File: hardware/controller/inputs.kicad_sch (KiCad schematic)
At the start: 19 parts, among them SW1 EVP-ASAC1A, SW2 EVP-ASAC1A, SW3 EVP-ASAC1A, SW4 EVP-ASAC1A, SW5 EVP-ASAC1A, SW6 CL-SB-13A-02T

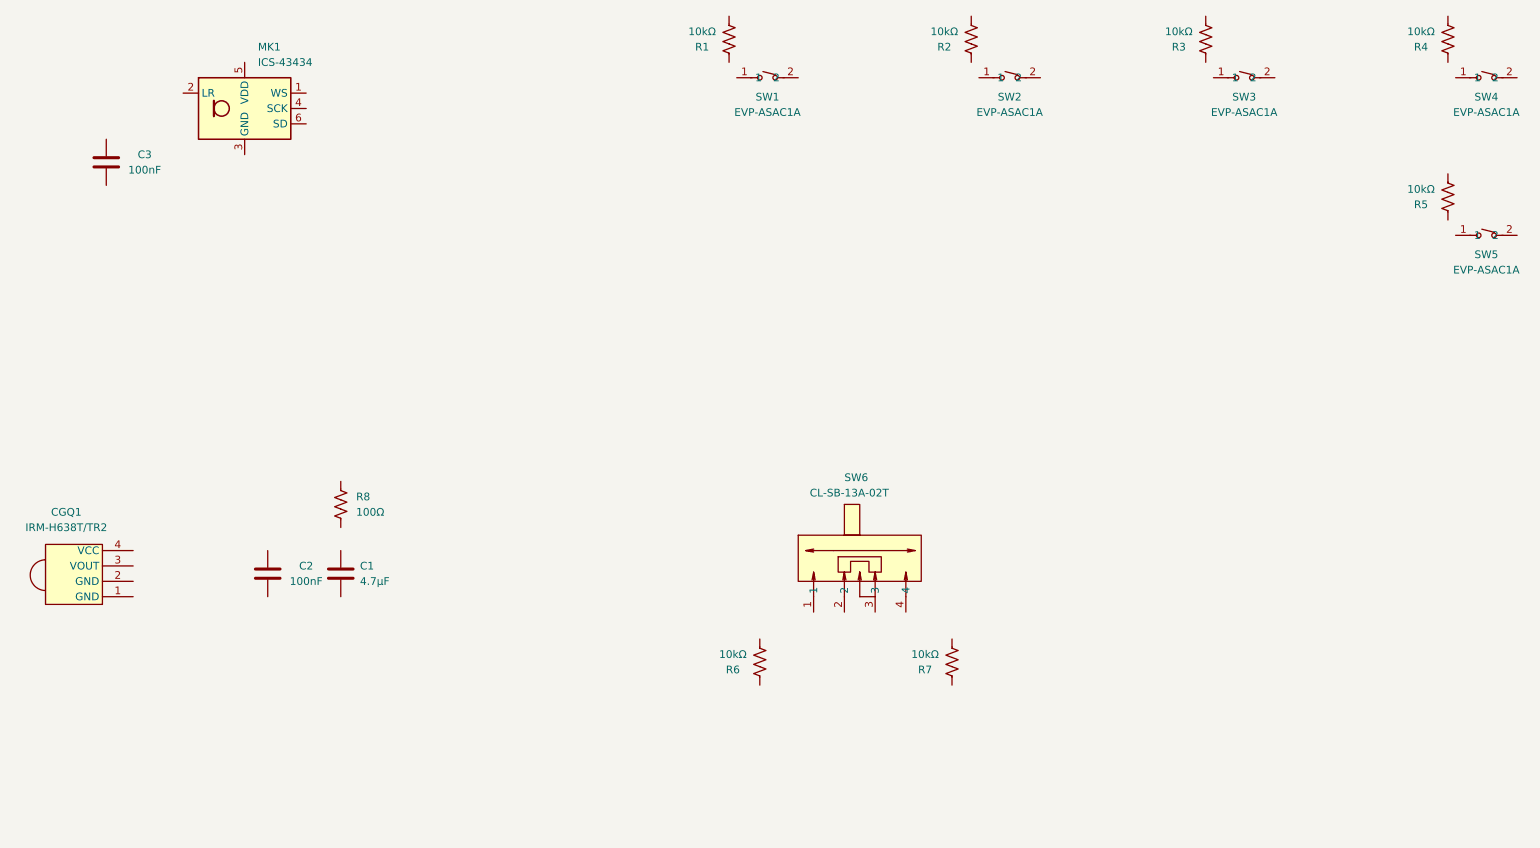
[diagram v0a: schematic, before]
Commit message: hooking up parts in the schematic
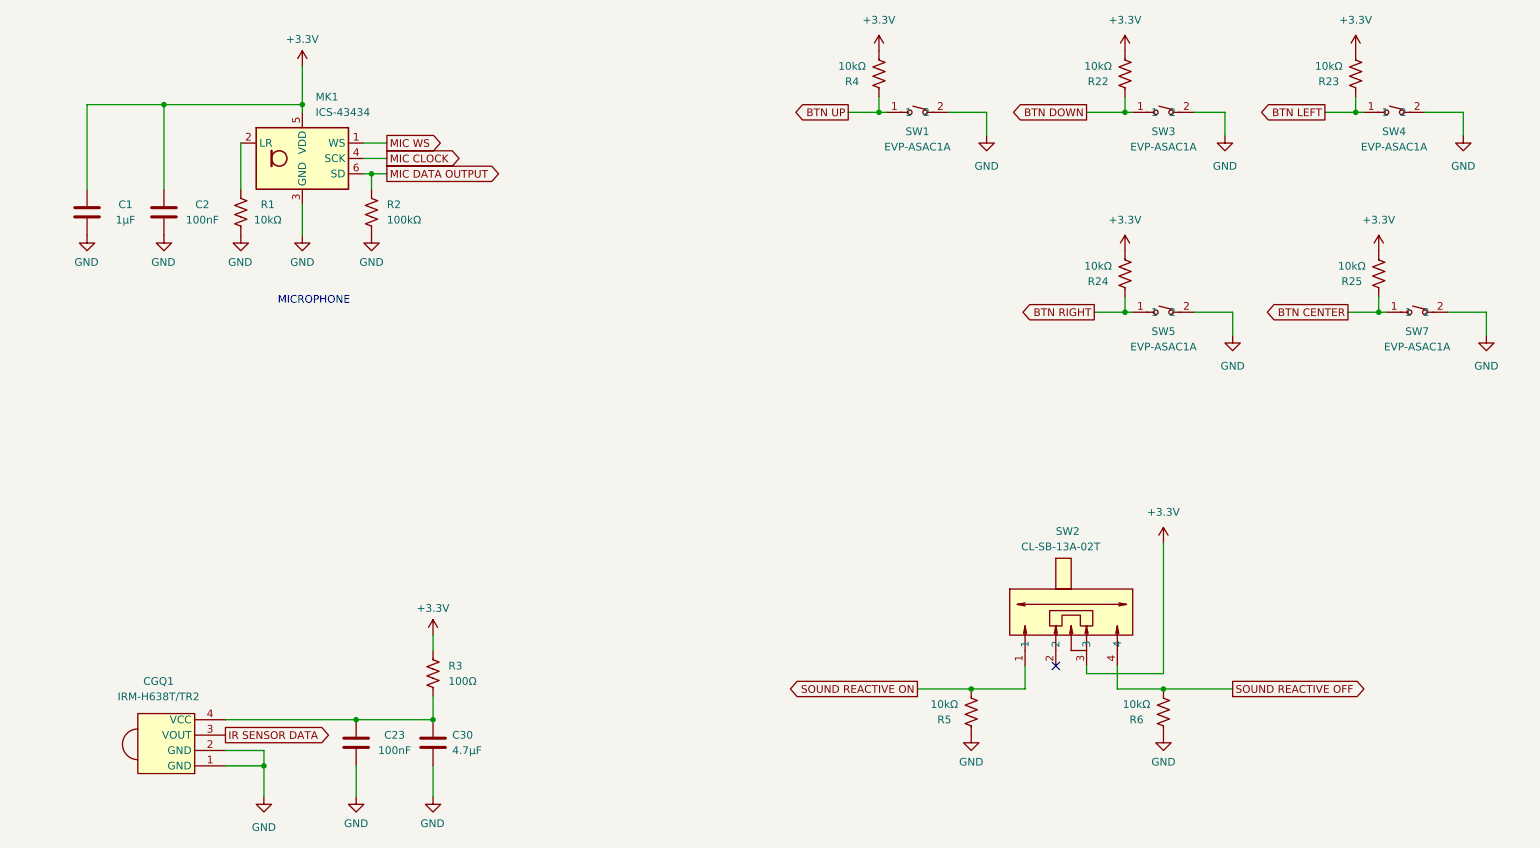
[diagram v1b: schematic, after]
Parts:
- removed C3: 100nF, Capacitor_SMD:C_0402_1005Metric, symbol Device:C
- removed R7: 10kΩ, Resistor_SMD:R_0402_1005Metric, symbol Device:R_US
- removed R8: 100Ω, Resistor_SMD:R_0402_1005Metric, symbol Device:R_US
- removed SW2: EVP-ASAC1A, easyeda2kicad:SW-SMD_PANASONIC_EVPASXXX, symbol easyeda2kicad:EVP-ASAC1A
- removed SW6: CL-SB-13A-02T, easyeda2kicad:SW-SMD_CL-SB-13A-0X, symbol easyeda2kicad:CL-SB-13A-02T
- added C23: 100nF, Capacitor_SMD:C_0402_1005Metric, symbol Device:C
- added C30: 4.7µF, Capacitor_SMD:C_0402_1005Metric, symbol Device:C
- added R22, R23, R24, R25: 10kΩ, Resistor_SMD:R_0402_1005Metric, symbol Device:R_US
- added SW2: CL-SB-13A-02T, easyeda2kicad:SW-SMD_CL-SB-13A-0X, symbol easyeda2kicad:CL-SB-13A-02T
- added SW7: EVP-ASAC1A, easyeda2kicad:SW-SMD_PANASONIC_EVPASXXX, symbol easyeda2kicad:EVP-ASAC1A
- C1: value 4.7µF -> 1µF; LCSC Part C23733 -> C52923
- R2: value 10kΩ -> 100kΩ; LCSC Part C25744 -> C60491
- R3: value 10kΩ -> 100Ω; LCSC Part C25744 -> C25076
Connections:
- net GND: now reaches CGQ1.1 (GND)
- net GND: now also C1.2, C2.2, CGQ1.2 (GND), MK1.3 (GND), R1.1, R2.1, R5.2, R6.2, SW1.2, SW3.2, SW4.2, SW5.2, C23.2, C30.1, SW7.2
- net IR SENSOR DATA: now reaches CGQ1.3 (VOUT)
- net at CGQ1.4 (VCC): now also R3.1, C23.1, C30.2
- net SOUND REACTIVE OFF: now reaches R6.1
- net SOUND REACTIVE OFF: now also SW2.4
- net BTN DOWN: now reaches SW3.1
- net BTN DOWN: now also R22.2
- net BTN UP: now reaches SW1.1
- net BTN UP: now also R4.2
- net MIC DATA OUTPUT: now reaches R2.2
- net MIC DATA OUTPUT: now also MK1.6 (SD)
- net BTN LEFT: now reaches SW4.1
- net BTN LEFT: now also R23.2
- net +3.3V: now reaches C2.1
- net +3.3V: now also C1.1, MK1.5 (VDD), R3.2, R4.1, R22.1, R23.1, R24.1, R25.1, SW2.3
- net MIC WS: now reaches MK1.1 (WS)
- net at MK1.2 (LR): now also R1.2
- net MIC CLOCK: now reaches MK1.4 (SCK)
- net BTN RIGHT: now reaches SW5.1
- net BTN RIGHT: now also R24.2
- net SOUND REACTIVE ON: now reaches R5.1
- net SOUND REACTIVE ON: now also SW2.1
- new net BTN CENTER: R25.2, SW7.1
- no-connect marks 0 -> 1
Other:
- note added: "MICROPHONE"
